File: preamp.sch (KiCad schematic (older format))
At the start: 2 parts

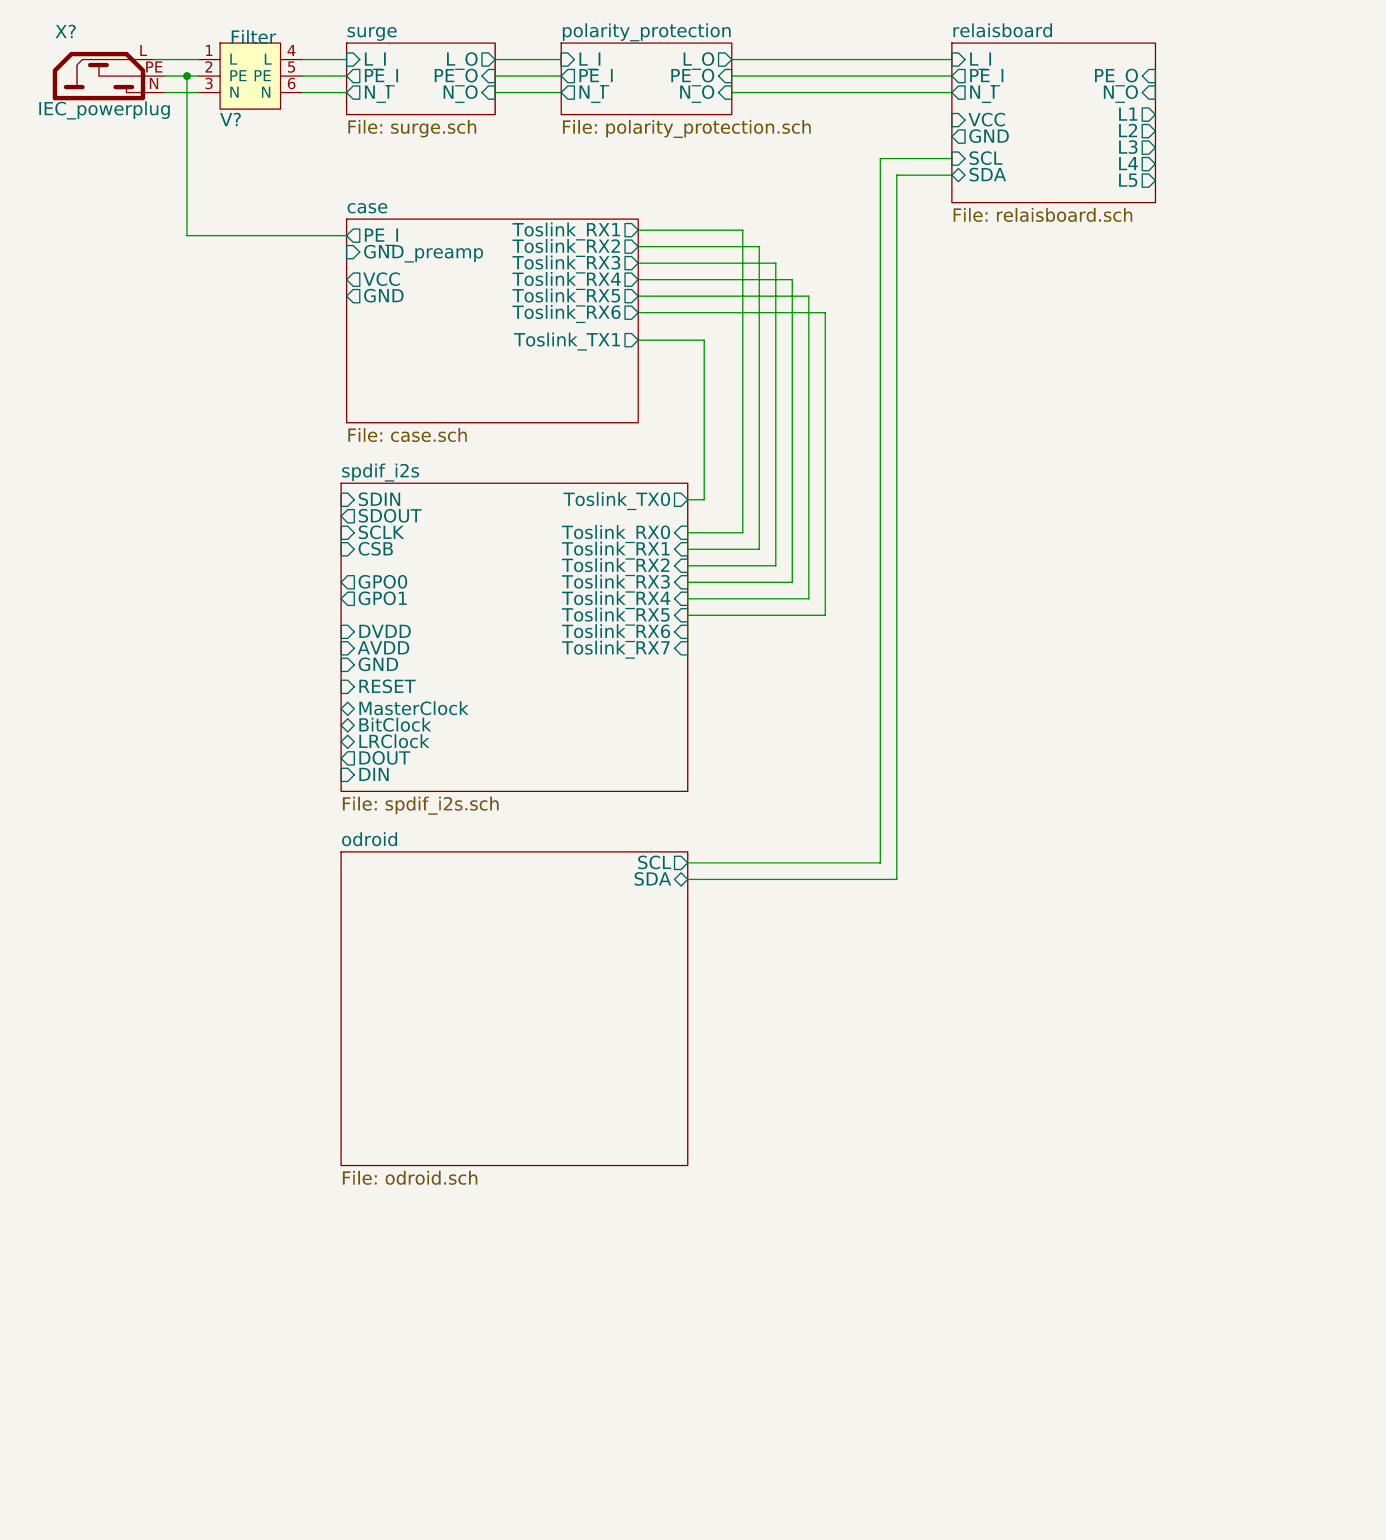
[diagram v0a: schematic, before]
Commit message: no idea what to write.
something :-D
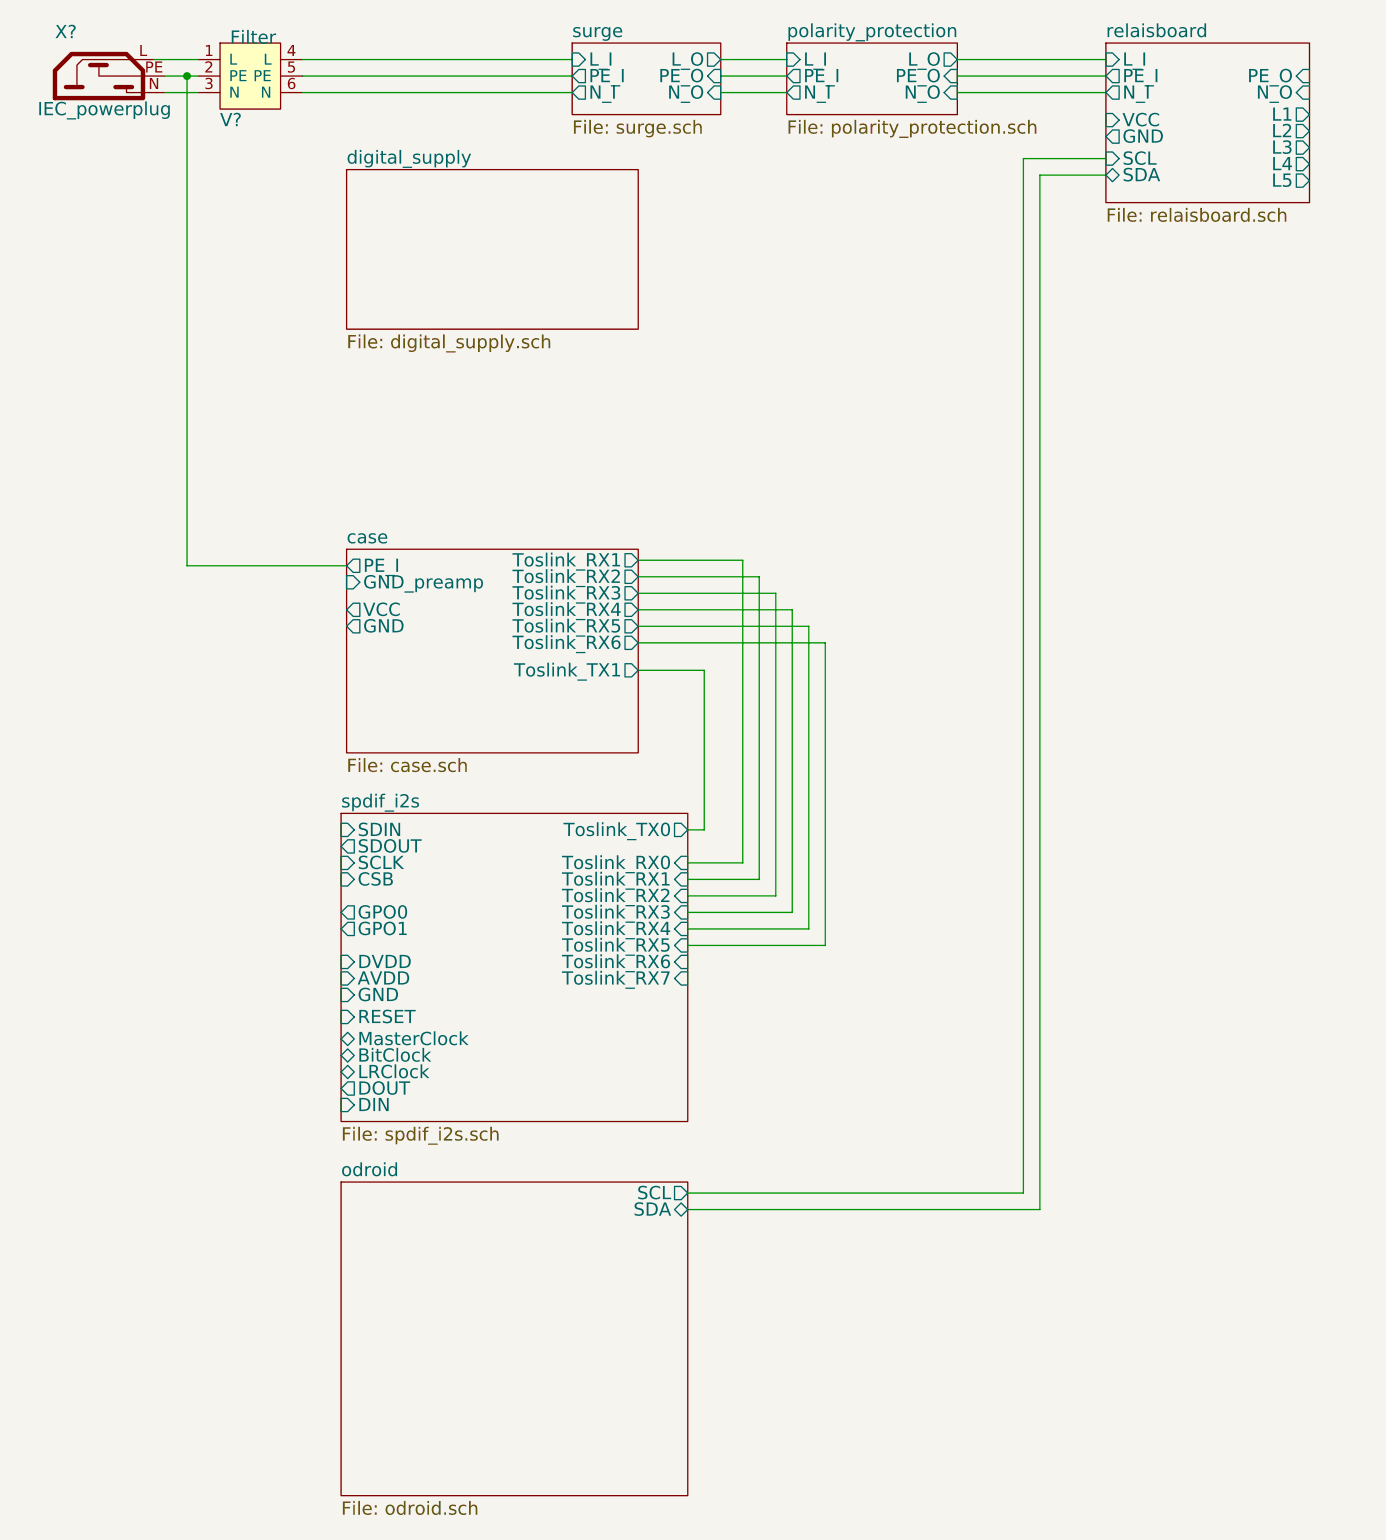
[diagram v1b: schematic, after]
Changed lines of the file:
@@
 $Descr A4 11693 8268
 encoding utf-8
-Sheet 1 7
+Sheet 1 8
 Title ""
 Date ""
@@
 $EndDescr
 $Sheet
-S 2000 825  675  325
+S 3025 825  675  325
 U 5882A13F
 F0 "surge" 60
 F1 "surge.sch" 60
-F2 "L_I" I L 2000 900 60
-F3 "PE_I" O L 2000 975 60
-F4 "N_I" O L 2000 1050 60
-F5 "L_O" O R 2675 900 60
-F6 "PE_O" I R 2675 975 60
-F7 "N_O" I R 2675 1050 60
+F2 "L_I" I L 3025 900 60
+F3 "PE_I" O L 3025 975 60
+F4 "N_I" O L 3025 1050 60
+F5 "L_O" O R 3700 900 60
+F6 "PE_O" I R 3700 975 60
+F7 "N_O" I R 3700 1050 60
 $EndSheet
 $Comp
@@
 $EndComp
 $Sheet
-S 2975 825  775  325
+S 4000 825  775  325
 U 58836B99
 F0 "polarity_protection" 60
 F1 "polarity_protection.sch" 60
-F2 "L_I" I L 2975 900 60
-F3 "PE_I" O L 2975 975 60
-F4 "N_I" O L 2975 1050 60
-F5 "L_O" O R 3750 900 60
-F6 "PE_O" I R 3750 975 60
-F7 "N_O" I R 3750 1050 60
-$EndSheet
-Wire Wire Line
-	2675 900  2975 900
-Wire Wire Line
-	2975 975  2675 975
-Wire Wire Line
-	2675 1050 2975 1050
-$Sheet
-S 4750 825  925  725
+F2 "L_I" I L 4000 900 60
+F3 "PE_I" O L 4000 975 60
+F4 "N_I" O L 4000 1050 60
+F5 "L_O" O R 4775 900 60
+F6 "PE_O" I R 4775 975 60
+F7 "N_O" I R 4775 1050 60
+$EndSheet
+Wire Wire Line
+	3700 900  4000 900
+Wire Wire Line
+	4000 975  3700 975
+Wire Wire Line
+	3700 1050 4000 1050
+$Sheet
+S 5450 825  925  725
 U 58838AD0
 F0 "relaisboard" 60
 F1 "relaisboard.sch" 60
-F2 "L_I" I L 4750 900 60
-F3 "PE_I" O L 4750 975 60
-F4 "N_I" O L 4750 1050 60
-F5 "PE_O" I R 5675 975 60
-F6 "N_O" I R 5675 1050 60
-F7 "L1" O R 5675 1150 60
-F8 "L2" O R 5675 1225 60
-F9 "L3" O R 5675 1300 60
-F10 "L4" O R 5675 1375 60
-F11 "L5" O R 5675 1450 60
-F12 "GND" O L 4750 1250 60
-F13 "VCC" I L 4750 1175 60
-F14 "SCL" I L 4750 1350 60
-F15 "SDA" B L 4750 1425 60
-$EndSheet
-Wire Wire Line
-	4750 900  3750 900
-Wire Wire Line
-	3750 975  4750 975
-Wire Wire Line
-	4750 1050 3750 1050
-$Sheet
-S 2000 1625 1325 925
+F2 "L_I" I L 5450 900 60
+F3 "PE_I" O L 5450 975 60
+F4 "N_I" O L 5450 1050 60
+F5 "PE_O" I R 6375 975 60
+F6 "N_O" I R 6375 1050 60
+F7 "L1" O R 6375 1150 60
+F8 "L2" O R 6375 1225 60
+F9 "L3" O R 6375 1300 60
+F10 "L4" O R 6375 1375 60
+F11 "L5" O R 6375 1450 60
+F12 "GND" O L 5450 1250 60
+F13 "VCC" I L 5450 1175 60
+F14 "SCL" I L 5450 1350 60
+F15 "SDA" B L 5450 1425 60
+$EndSheet
+Wire Wire Line
+	5450 900  4775 900
+Wire Wire Line
+	4775 975  5450 975
+Wire Wire Line
+	5450 1050 4775 1050
+$Sheet
+S 2000 3125 1325 925
 U 5883E969
 F0 "case" 60
 F1 "case.sch" 60
-F2 "GND_preamp" I L 2000 1775 60
-F3 "PE_I" O L 2000 1700 60
-F4 "GND" O L 2000 1975 60
-F5 "VCC" O L 2000 1900 60
-F6 "Toslink_RX1" O R 3325 1675 60
-F7 "Toslink_RX2" O R 3325 1750 60
-F8 "Toslink_RX3" O R 3325 1825 60
-F9 "Toslink_RX4" O R 3325 1900 60
-F10 "Toslink_RX5" O R 3325 1975 60
-F11 "Toslink_RX6" O R 3325 2050 60
-F12 "Toslink_TX1" O R 3325 2175 60
-$EndSheet
-$Sheet
-S 1975 4500 1575 1425
+F2 "GND_preamp" I L 2000 3275 60
+F3 "PE_I" O L 2000 3200 60
+F4 "GND" O L 2000 3475 60
+F5 "VCC" O L 2000 3400 60
+F6 "Toslink_RX1" O R 3325 3175 60
+F7 "Toslink_RX2" O R 3325 3250 60
+F8 "Toslink_RX3" O R 3325 3325 60
+F9 "Toslink_RX4" O R 3325 3400 60
+F10 "Toslink_RX5" O R 3325 3475 60
+F11 "Toslink_RX6" O R 3325 3550 60
+F12 "Toslink_TX1" O R 3325 3675 60
+$EndSheet
+$Sheet
+S 1975 6000 1575 1425
 U 58843538
 F0 "odroid" 60
 F1 "odroid.sch" 60
-F2 "SCL" O R 3550 4550 60
-F3 "SDA" B R 3550 4625 60
-$EndSheet
-$Sheet
-S 1975 2825 1575 1400
+F2 "SCL" O R 3550 6050 60
+F3 "SDA" B R 3550 6125 60
+$EndSheet
+$Sheet
+S 1975 4325 1575 1400
 U 5885CB61
 F0 "spdif_i2s" 60
 F1 "spdif_i2s.sch" 60
-F2 "RESET" I L 1975 3750 60
-F3 "SDOUT" O L 1975 2975 60
-F4 "SDIN" I L 1975 2900 60
-F5 "SCLK" I L 1975 3050 60
-F6 "CSB" I L 1975 3125 60
-F7 "GPO1" O L 1975 3350 60
-F8 "GPO0" O L 1975 3275 60
-F9 "Toslink_TX0" O R 3550 2900 60
-F10 "Toslink_RX7" I R 3550 3575 60
-F11 "Toslink_RX6" I R 3550 3500 60
-F12 "Toslink_RX5" I R 3550 3425 60
-F13 "Toslink_RX4" I R 3550 3350 60
-F14 "Toslink_RX3" I R 3550 3275 60
-F15 "Toslink_RX2" I R 3550 3200 60
-F16 "Toslink_RX1" I R 3550 3125 60
-F17 "Toslink_RX0" I R 3550 3050 60
-F18 "MasterClock" B L 1975 3850 60
-F19 "BitClock" B L 1975 3925 60
-F20 "LRClock" B L 1975 4000 60
-F21 "DOUT" O L 1975 4075 60
-F22 "DIN" I L 1975 4150 60
-F23 "DVDD" I L 1975 3500 60
-F24 "AVDD" I L 1975 3575 60
-F25 "GND" I L 1975 3650 60
+F2 "RESET" I L 1975 5250 60
+F3 "SDOUT" O L 1975 4475 60
+F4 "SDIN" I L 1975 4400 60
+F5 "SCLK" I L 1975 4550 60
+F6 "CSB" I L 1975 4625 60
+F7 "GPO1" O L 1975 4850 60
+F8 "GPO0" O L 1975 4775 60
+F9 "Toslink_TX0" O R 3550 4400 60
+F10 "Toslink_RX7" I R 3550 5075 60
+F11 "Toslink_RX6" I R 3550 5000 60
+F12 "Toslink_RX5" I R 3550 4925 60
+F13 "Toslink_RX4" I R 3550 4850 60
+F14 "Toslink_RX3" I R 3550 4775 60
+F15 "Toslink_RX2" I R 3550 4700 60
+F16 "Toslink_RX1" I R 3550 4625 60
+F17 "Toslink_RX0" I R 3550 4550 60
+F18 "MasterClock" B L 1975 5350 60
+F19 "BitClock" B L 1975 5425 60
+F20 "LRClock" B L 1975 5500 60
+F21 "DOUT" O L 1975 5575 60
+F22 "DIN" I L 1975 5650 60
+F23 "DVDD" I L 1975 5000 60
+F24 "AVDD" I L 1975 5075 60
+F25 "GND" I L 1975 5150 60
 $EndSheet
 $Comp
@@
 	1325 900  1125 900
 Wire Wire Line
-	1175 975  1275 975
-Wire Wire Line
-	1275 975  1325 975
+	1175 975  1325 975
 Wire Wire Line
 	1175 1050 1325 1050
 Wire Wire Line
-	1800 900  2000 900
-Wire Wire Line
-	1800 975  2000 975
-Wire Wire Line
-	1800 1050 2000 1050
-Wire Wire Line
-	2000 1700 1275 1700
-Wire Wire Line
-	1275 1700 1275 975
+	1800 900  3025 900
+Wire Wire Line
+	1800 975  3025 975
+Wire Wire Line
+	1800 1050 3025 1050
+Wire Wire Line
+	2000 3200 1275 3200
+Wire Wire Line
+	1275 3200 1275 975
 Connection ~ 1275 975
 Wire Wire Line
-	3325 2175 3625 2175
-Wire Wire Line
-	3625 2175 3625 2900
-Wire Wire Line
-	3625 2900 3550 2900
-Wire Wire Line
-	3550 3050 3800 3050
-Wire Wire Line
-	3800 3050 3800 1675
-Wire Wire Line
-	3800 1675 3325 1675
-Wire Wire Line
-	3550 3125 3875 3125
-Wire Wire Line
-	3875 3125 3875 1750
-Wire Wire Line
-	3875 1750 3325 1750
-Wire Wire Line
-	3325 1825 3950 1825
-Wire Wire Line
-	3950 1825 3950 3200
-Wire Wire Line
-	3950 3200 3550 3200
-Wire Wire Line
-	3550 3275 4025 3275
-Wire Wire Line
-	4025 3275 4025 1900
-Wire Wire Line
-	4025 1900 3325 1900
-Wire Wire Line
-	3325 1975 4100 1975
-Wire Wire Line
-	4100 1975 4100 3350
-Wire Wire Line
-	4100 3350 3550 3350
-Wire Wire Line
-	3550 3425 4175 3425
-Wire Wire Line
-	4175 3425 4175 2050
-Wire Wire Line
-	4175 2050 3325 2050
-Wire Wire Line
-	3550 4550 4425 4550
-Wire Wire Line
-	4425 4550 4425 1350
-Wire Wire Line
-	4425 1350 4750 1350
-Wire Wire Line
-	3550 4625 4500 4625
-Wire Wire Line
-	4500 4625 4500 1425
-Wire Wire Line
-	4500 1425 4750 1425
+	3325 3675 3625 3675
+Wire Wire Line
+	3625 3675 3625 4400
+Wire Wire Line
+	3625 4400 3550 4400
+Wire Wire Line
+	3550 4550 3800 4550
+Wire Wire Line
+	3800 4550 3800 3175
+Wire Wire Line
+	3800 3175 3325 3175
+Wire Wire Line
+	3550 4625 3875 4625
+Wire Wire Line
+	3875 4625 3875 3250
+Wire Wire Line
+	3875 3250 3325 3250
+Wire Wire Line
+	3325 3325 3950 3325
+Wire Wire Line
+	3950 3325 3950 4700
+Wire Wire Line
+	3950 4700 3550 4700
+Wire Wire Line
+	3550 4775 4025 4775
+Wire Wire Line
+	4025 4775 4025 3400
+Wire Wire Line
+	4025 3400 3325 3400
+Wire Wire Line
+	3325 3475 4100 3475
+Wire Wire Line
+	4100 3475 4100 4850
+Wire Wire Line
+	4100 4850 3550 4850
+Wire Wire Line
+	3550 4925 4175 4925
+Wire Wire Line
+	4175 4925 4175 3550
+Wire Wire Line
+	4175 3550 3325 3550
+Wire Wire Line
+	3550 6050 5075 6050
+Wire Wire Line
+	5075 6050 5075 1350
+Wire Wire Line
+	5075 1350 5450 1350
+Wire Wire Line
+	3550 6125 5150 6125
+Wire Wire Line
+	5150 6125 5150 1425
+Wire Wire Line
+	5150 1425 5450 1425
+$Sheet
+S 2000 1400 1325 725
+U 58A1535E
+F0 "digital_supply" 60
+F1 "digital_supply.sch" 60
+$EndSheet
 $EndSCHEMATC
